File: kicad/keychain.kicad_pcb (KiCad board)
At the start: 2 copper layers, 68.1 x 37.9 mm, 60 parts, among them J1 USB-C, J2 LiPo, J3 FPC-SMD_FH34SRJ-26S-0.5SH-50, Q1 BSS138, Q2 AO3401A, Q3 S8050, SW1 PWR, SW2 BOOT, SW3 USER, U1 ESP32-C6-MINI-1, U2 MCP73831, U3 AP2112K-3.3

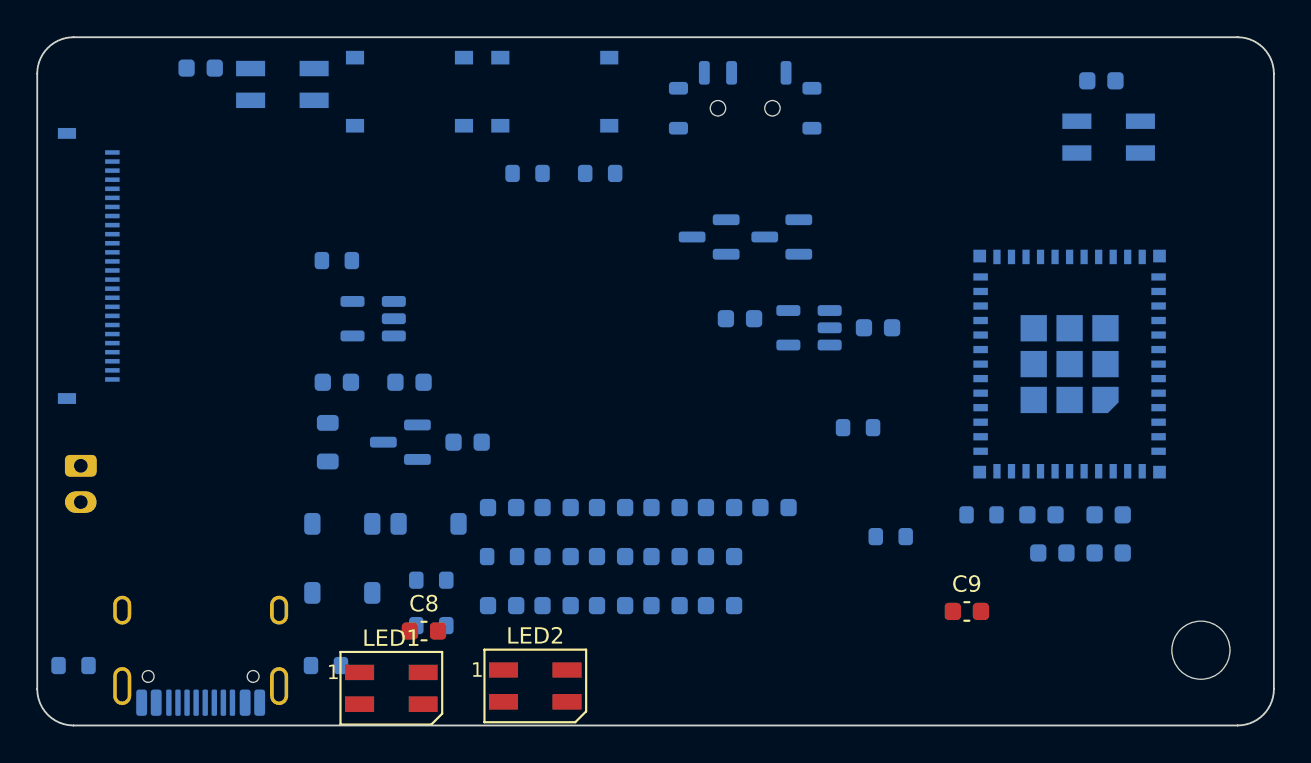
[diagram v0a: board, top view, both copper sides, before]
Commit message: Route board: freerouting SES + direct-link fixes, GND zones F/B, 0 unrouted
Generated with [Devin](https://devin.ai)

Co-Authored-By: Devin <158243242+devin-ai-integration[bot]@users.noreply.github.com>
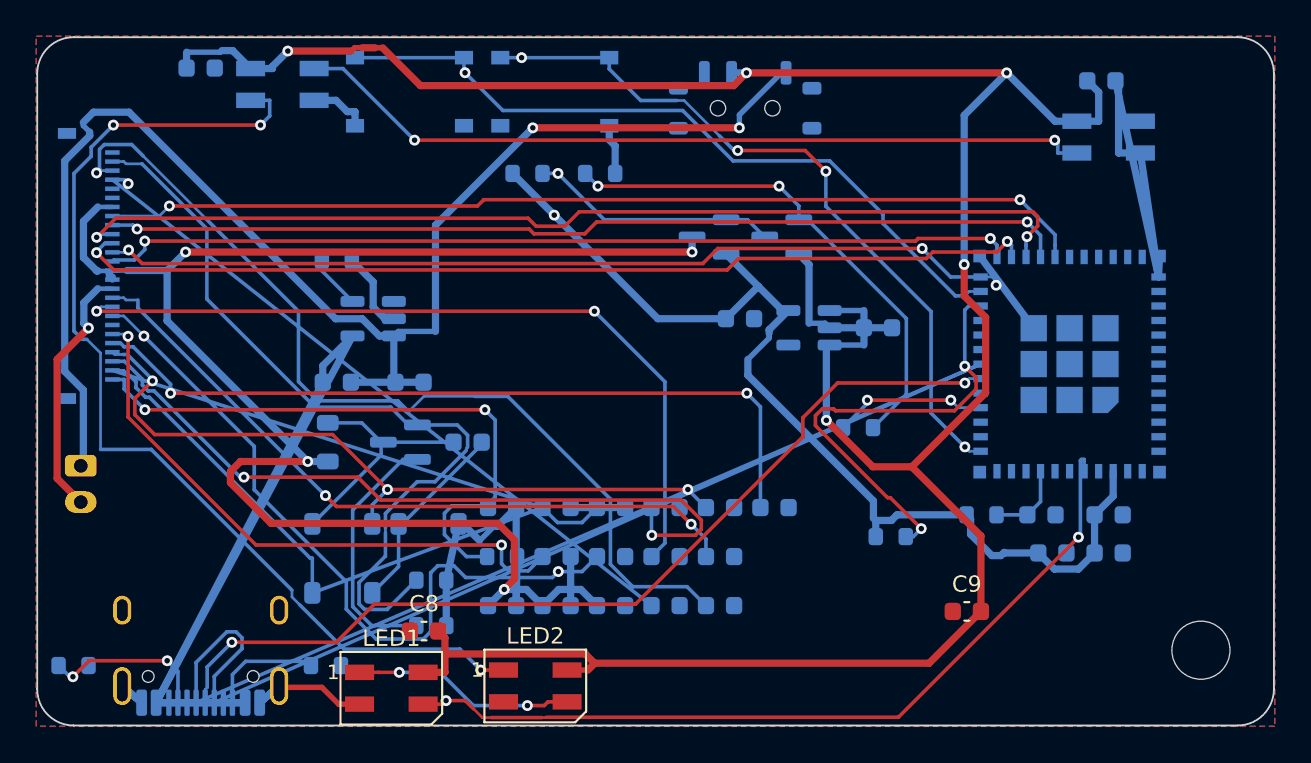
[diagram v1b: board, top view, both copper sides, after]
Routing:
- net /VBAT_SW: track 0.00 -> 143.9 mm, vias 0 -> 5
- net /USB_DP: track 0.00 -> 103.0 mm
- net GND: track 0.00 -> 101.1 mm, vias 0 -> 1
- net /VCC: track 0.00 -> 86.9 mm, vias 0 -> 4
- net +BATT: track 0.00 -> 76.6 mm, vias 0 -> 2
- net /EPD_VGL: track 0.00 -> 59.5 mm
- net +3V3: track 0.00 -> 57.9 mm, vias 0 -> 1
- net /LED_C2: track 0.00 -> 57.7 mm, vias 0 -> 3
- net /EPD_DC: track 0.00 -> 56.3 mm, vias 0 -> 2
- net VBUS: track 0.00 -> 55.8 mm
- net /EPD_BUSY: track 0.00 -> 54.3 mm, vias 0 -> 2
- net /EPD_CS: track 0.00 -> 53.3 mm, vias 0 -> 2
- net /EPD_RST: track 0.00 -> 53.1 mm, vias 0 -> 2
- net /USB_DM: track 0.00 -> 52.8 mm, vias 0 -> 2
- net /EPD_TVCOM: track 0.00 -> 51.2 mm, vias 0 -> 1
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- added copper zone on B.Cu, net GND
- added copper zone on F.Cu, net GND
